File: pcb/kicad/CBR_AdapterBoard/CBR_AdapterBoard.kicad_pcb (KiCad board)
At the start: 2 copper layers, 80 x 46.3 mm, 7 parts, among them J1 2125201004, J2 2125201004, J3 2125201004, J4 2125201004, J5 2125201004, J6 2125201004, J7 AJK_22_Pin

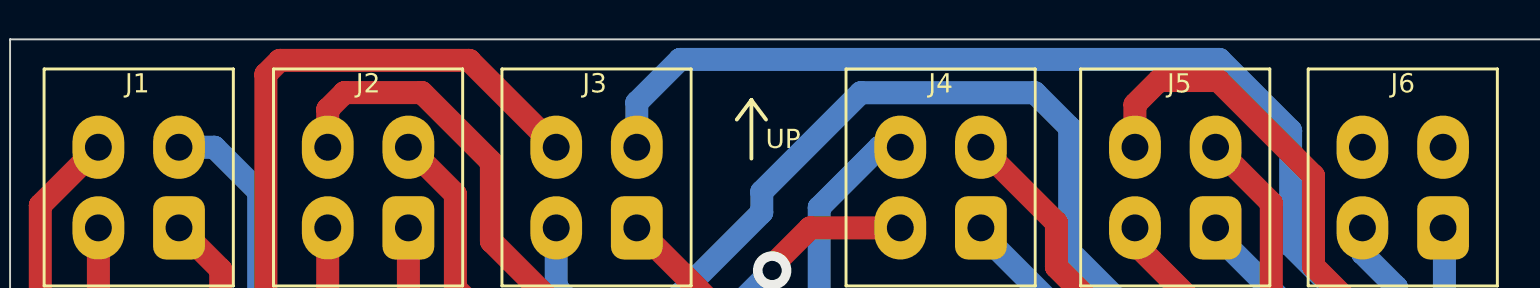
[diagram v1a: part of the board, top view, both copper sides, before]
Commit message: - File corrections.
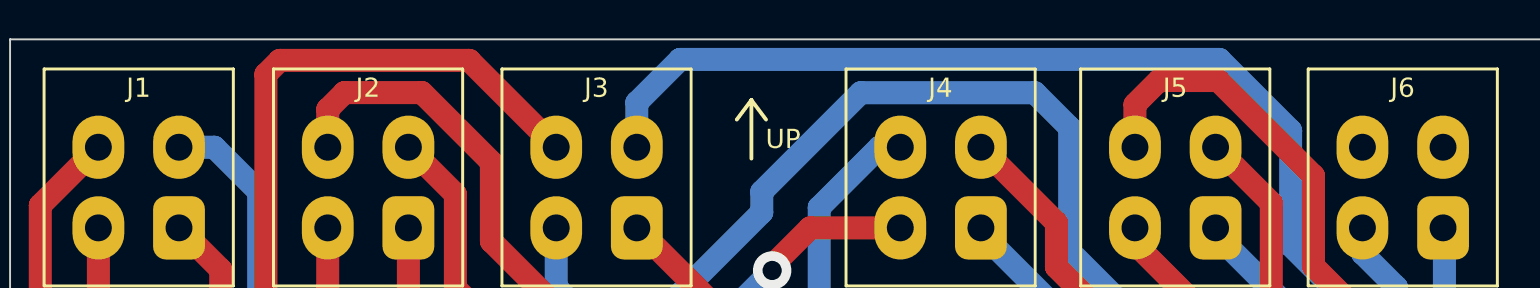
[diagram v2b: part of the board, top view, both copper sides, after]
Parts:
- J1, J2, J3, J4, J5, J6: footprint AJK_MolexPin:4-Way-Molex_Connector-MiniFit-JNR -> Blackbird:4-Way-Molex_Connector-MiniFit-JNR
- J7: value AJK_22_Pin -> Keihin_22_Pin; footprint AJK_MolexPin:AJK_Single_MolexPin_1.8mmHole -> Blackbird:Blackbird_22_pin_keihin
